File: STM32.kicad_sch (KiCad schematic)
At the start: 13 parts

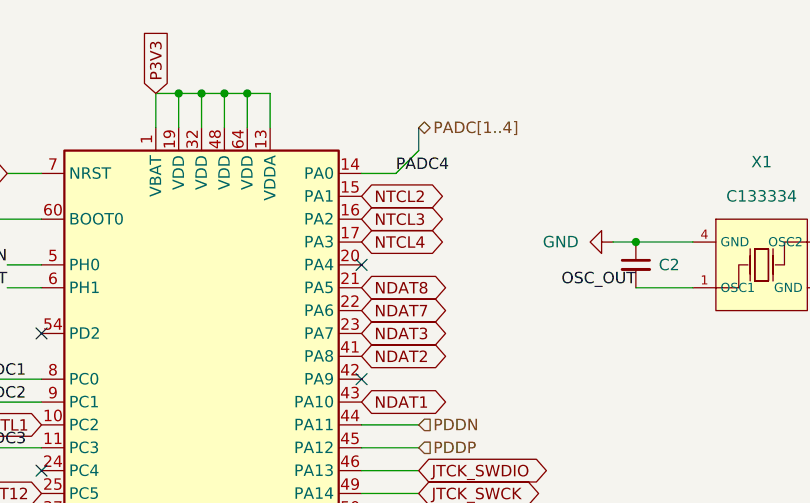
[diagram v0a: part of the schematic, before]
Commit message: JLINK will complite
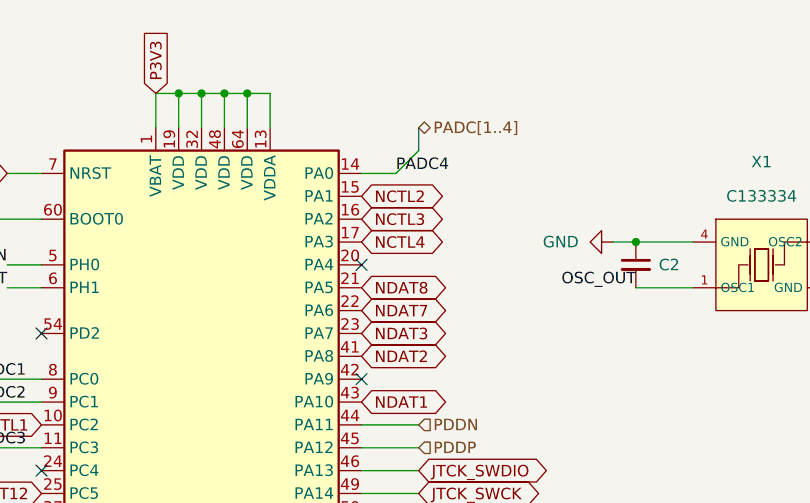
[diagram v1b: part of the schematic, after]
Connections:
- net NTCL2 renamed NCTL2
- net NTCL3 renamed NCTL3
- net NTCL4 renamed NCTL4
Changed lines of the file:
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@@
 		)
 	)
-	(global_label "NTCL3"
+	(global_label "NCTL3"
 		(shape bidirectional)
 		(at 109.22 73.66 0)
@@
 		)
 	)
-	(global_label "NTCL4"
+	(global_label "NCTL4"
 		(shape bidirectional)
 		(at 109.22 76.2 0)
@@
 		)
 	)
-	(global_label "NTCL2"
+	(global_label "NCTL2"
 		(shape bidirectional)
 		(at 109.22 71.12 0)
